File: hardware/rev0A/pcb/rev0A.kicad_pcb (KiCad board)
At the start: 2 copper layers, 95 x 75 mm, 83 parts, among them IC1 ESP32-C3-WROOM-02-H4, IC2 TXS0102DCU, J1 Conn_01x02_Socket, J2 Conn_01x02_Socket, J3 Conn_01x02_Socket, J4 Conn_01x03_Socket, J5 Conn_01x02_Socket, J7 Conn_01x06_Socket, K1 SRD-12VDC-SL-C, K2 SRD-12VDC-SL-C, K3 SRD-12VDC-SL-C, Q1 BC337, Q2 BC337, Q3 BC337, SW1 SW_Push, SW2 SW_Push, U1 ADS1115IRUGT

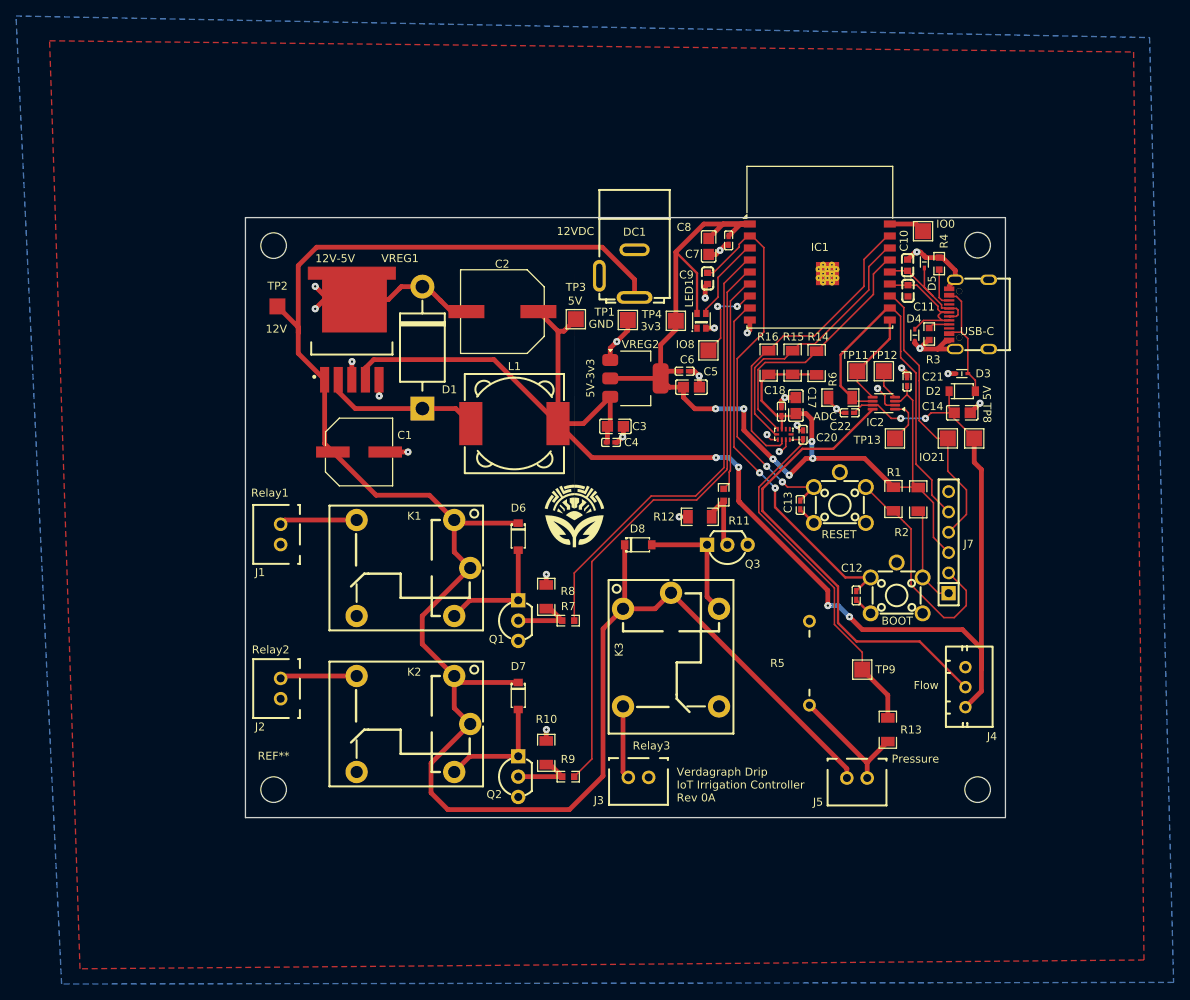
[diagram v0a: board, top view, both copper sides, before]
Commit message: Rev0A of the PCB
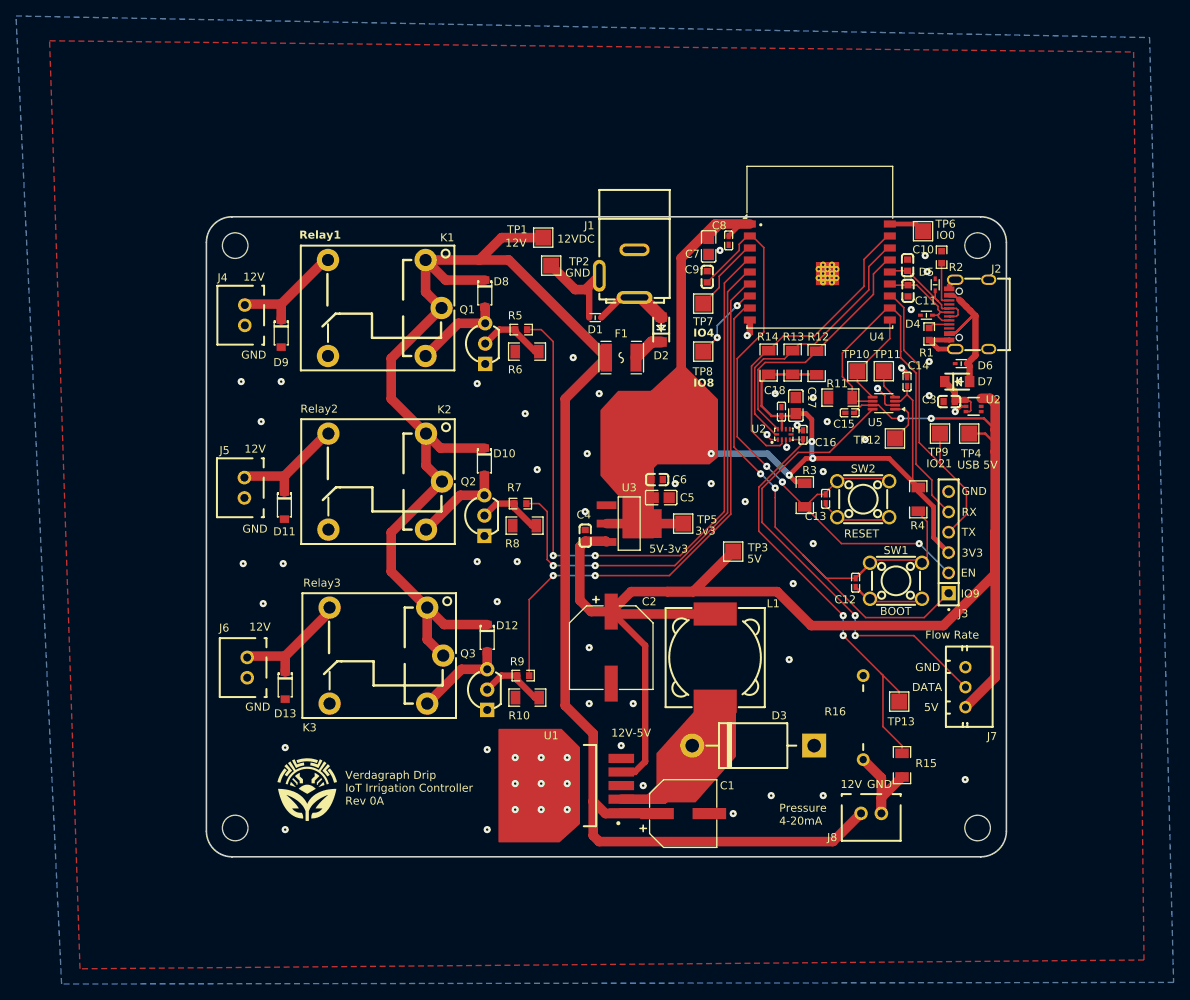
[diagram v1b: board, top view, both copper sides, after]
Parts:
- removed the C3 at (151.5, 87.6)
- removed DC1: EJ508A, easyeda2kicad:DC-IN-TH_EJ508A
- removed LED1: WS2812B-2020, easyeda2kicad:LED-SMD_4P-L2.0-W2.0-TL_WS2812B-2020
- removed VREG2: AMS1117, Package_TO_SOT_SMD:SOT-223-3_TabPin2
- added D1: LESD5D5.0CT1G, easyeda2kicad:SOD-523_L1.2-W0.8-LS1.6-BI, F.Cu at (149.0, 74.0)
- added D11: 1N4148W, easyeda2kicad:SOD-123_L2.8-W1.8-LS3.7-RD, F.Cu at (110.2, 97.5)
- added D13: 1N4148W, easyeda2kicad:SOD-123_L2.8-W1.8-LS3.7-RD, F.Cu at (110.2, 120.0)
- added D2: MBR230LSFT1G, easyeda2kicad:SOD-123FL_L2.8-W1.8-LS3.6-RD, F.Cu at (157.2, 75.5)
- added D9: 1N4148W, easyeda2kicad:SOD-123_L2.8-W1.8-LS3.7-RD, F.Cu at (109.8, 76.0)
- added F1: 1A, easyeda2kicad:F1812, F.Cu at (152.2, 79.0)
- added J1: EJ508A, easyeda2kicad:DC-IN-TH_EJ508A, F.Cu at (151.7, 68.5)
- added TP7: ~, TestPoint:TestPoint_Pad_2.0x2.0mm, F.Cu at (162.5, 72.2)
- added U2: TPS22919QDCKRQ1, easyeda2kicad:SC-70-6_L2.0-W1.3-P0.65-LS2.1-BR, F.Cu at (196.3, 85.1)
- added U3: LDL1117S33R, easyeda2kicad:SOT-223-4_L6.5-W3.5-P2.30-LS7.0-BR, F.Cu at (153.2, 99.8)
- C2: footprint easyeda2kicad:CAP-SMD_BD10.0-L10.3-W10.3-FD -> easyeda2kicad:CAP-SMD_BD10.0-L10.3-W10.3-LS11.3-FD
- C3: renamed from C14; value 10uF -> 1uF; footprint easyeda2kicad:C0805 -> easyeda2kicad:C0603
- C4, C6: value 0.1uF -> 1uF; footprint easyeda2kicad:C0402 -> easyeda2kicad:C0603
- D7: renamed from D2; value 1N5819 -> MBR230LSFT1G; footprint easyeda2kicad:SOD-123_L2.7-W1.6-LS3.7-RD -> easyeda2kicad:SOD-123FL_L2.8-W1.8-LS3.6-RD
- J3: renamed from J7; value Conn_01x06_Socket -> 6 Pin Socket Header
- J4: renamed from J1; value Conn_01x02_Socket -> 2 Pin JST
- J5: renamed from J2; value Conn_01x02_Socket -> 2 Pin JST
- J6: renamed from J3; value Conn_01x02_Socket -> 2 Pin JST
- J7: renamed from J4; value Conn_01x03_Socket -> 3 Pin JST
- J8: renamed from J5; value Conn_01x02_Socket -> 2 Pin JST
- SW1, SW2: footprint easyeda2kicad:SW-TH_5P-L6.0-W6.0-P4.50-LS6.5 -> easyeda2kicad:SW-TH_4P-L6.0-W6.0-P4.50-LS6.5
- moved D3 64.7 mm to (168.8, 127.5), turned to 180 degrees
- moved U1 62.7 mm to (147.2, 132.5), turned to 180 degrees
- moved C1 60.7 mm to (160.0, 136.0)
- moved J6 50.8 mm to (105.5, 117.8), turned to 90 degrees
- moved G*** 47.8 mm to (113.0, 133.0)
- moved C2 44.1 mm to (151.0, 115.2), turned to -90 degrees
- moved L1 38.5 mm to (164.0, 116.5), turned to 90 degrees
- moved R5 36.9 mm to (139.8, 75.5)
- moved K3 35.6 mm to (122.9, 116.2), turned to 180 degrees
- moved TP3 35.1 mm to (166.2, 103.2)
- moved Q3 35.1 mm to (135.5, 120.5), turned to 90 degrees
- moved Q1 34.9 mm to (135.2, 77.2)
- moved R7 34.6 mm to (139.7, 97.2)
- moved TP1 34.3 mm to (142.5, 64.0)
- moved R9 33.7 mm to (140.0, 118.8), turned to 180 degrees
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- renumbered C21 to C14, C22 to C15, C20 to C16, D7 to D10, D8 to D12, D1 to D3, D3 to D6, D6 to D8, USBC1 to J2, R3 to R1, R12 to R10, R6 to R11, R14 to R12, R15 to R13, R16 to R14, R13 to R15, R5 to R16, R4 to R2, R1 to R3, R2 to R4, R7 to R5, R8 to R6, R9 to R7, R10 to R8, R11 to R9, TP2 to TP1, TP11 to TP10, TP12 to TP11, TP13 to TP12, TP9 to TP13, TP1 to TP2, TP8 to TP4, TP4 to TP5, IO0 to TP6, IO8 to TP8, IO21 to TP9, VREG1 to U1, IC1 to U4, IC2 to U5, U1 to U6
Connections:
- net Pressure Sensor Voltage renamed Net-(U6-AIN0)
- C3 pad 1: +5V -> Net-(D7-K)
- C9 pad 1: GND -> CHIP_PU
- C9 pad 2: CHIP_PU -> GND
- D10 pad 2: Net-(D7-A) (its old number) -> Net-(D10-A)
- D12 pad 2: Net-(D8-A) -> Net-(D12-A)
- D3 pad 1: Net-(D1-K) -> GND
- D3 pad 2: GND -> Net-(D3-K)
- D7 pad 1: +5V -> Net-(D7-K)
- D8 pad 2: Net-(D6-A) -> Net-(D8-A)
- K1 pad C2: Net-(D6-A) -> Net-(D8-A)
- K2 pad C2: Net-(D7-A) (its old number) -> Net-(D10-A)
- K3 pad C2: Net-(D8-A) -> Net-(D12-A)
- L1 pad 1: Net-(D1-K) -> Net-(D3-K)
- Q1 pad 1: Net-(D6-A) -> GND
- Q1 pad 3: GND -> Net-(D8-A)
- Q2 pad 1: Net-(D7-A) (its old number) -> GND
- Q2 pad 3: GND -> Net-(D10-A)
- Q3 pad 1: Net-(D8-A) -> GND
- Q3 pad 3: GND -> Net-(D12-A)
- U1 pad 2: Net-(D1-K) -> Net-(D3-K)
- U4 pad 3: RGB -> Net-(U4-IO4)
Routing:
- net GND: track 113.9 -> 69.2 mm, vias 26 -> 62
- net Relay3: track 27.1 -> 69.1 mm, vias 0 -> 2
- net Relay1: track 57.6 -> 87.2 mm, vias 0 -> 2
- net GPIO9: track 59.0 -> 84.0 mm
- net Net-(D3-K): track 0.00 -> 20.2 mm
- net Net-(D1-K): track 19.7 -> 0.00 mm
- net Net-(D6-A): track 15.1 -> 0.00 mm
- net Net-(D7-A) (its old number): track 14.7 -> 0.00 mm
- net +12V: track 247.4 -> 234.2 mm
- net Net-(D10-A): track 0.00 -> 11.6 mm
- net Net-(D12-A): track 0.00 -> 11.5 mm
- net RGB: track 10.6 -> 0.00 mm
- net Net-(U6-AIN0): track 45.5 -> 55.1 mm, vias 0 -> 2
- net Net-(D2-A): track 0.00 -> 9.56 mm
- net Net-(U4-IO4): track 0.00 -> 9.54 mm
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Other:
- board size 95 x 75 mm -> 100 x 80 mm
- board text added: "3V3"
- board text added: "DATA"
- board text added: "EN"
- board text added: "Flow Rate"
- board text added: "IO0"
- board text added: "IO21"
- board text added: "IO4"
- board text added: "IO8"
- board text added: "IO9"
- board text added: "J2"
- board text added: "Pressure 4-20mA"
- board text added: "RX"
- board text added: "TX"
- board text added: "U2"
- board text added: "USB 5V"
- board text removed: "ADC"
- board text removed: "Flow"
- board text removed: "Pressure"
- board text removed: "USB-C"
